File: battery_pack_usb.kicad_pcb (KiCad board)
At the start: 2 copper layers, 30.4 x 15 mm, 25 parts, among them J1 Conn_01x02_Male, J2 USB_C_Receptacle_USB2.0, SW1 SW_SPST, U1 BQ25886

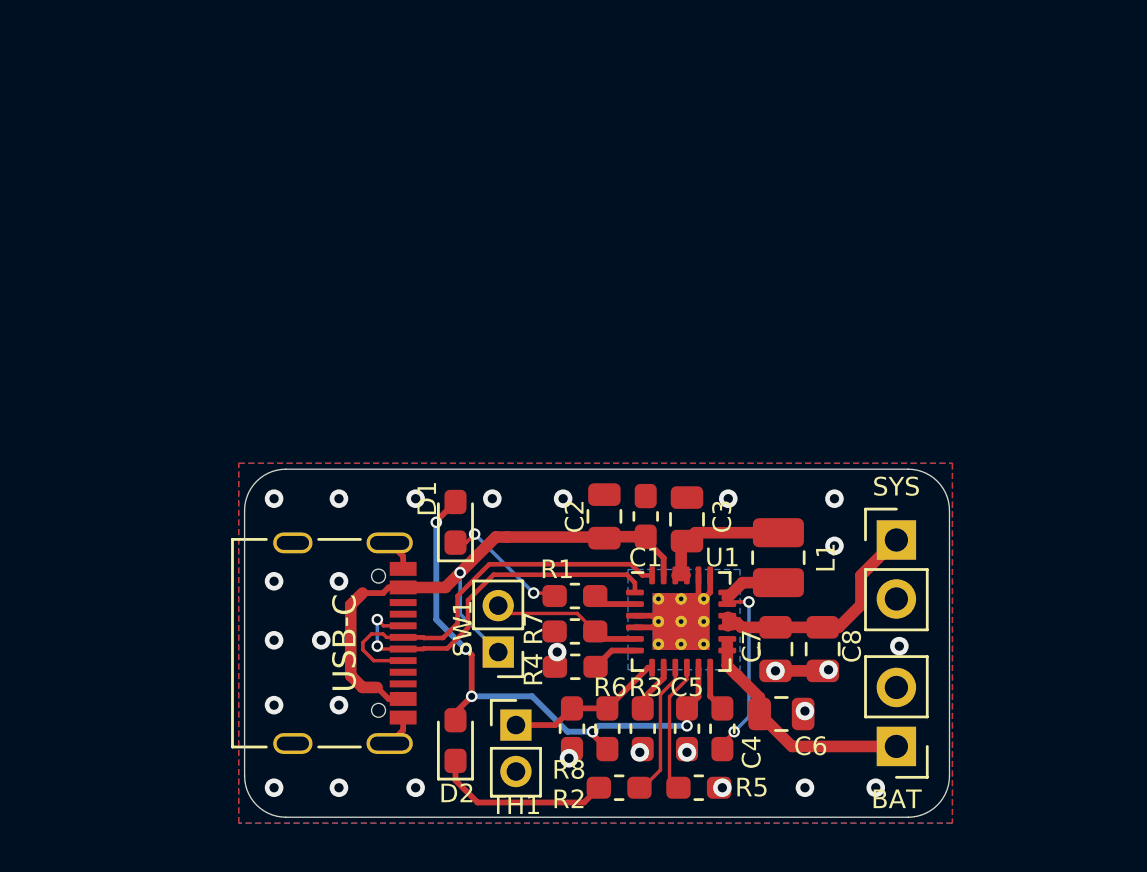
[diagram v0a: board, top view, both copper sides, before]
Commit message: Improve circuit and PCB
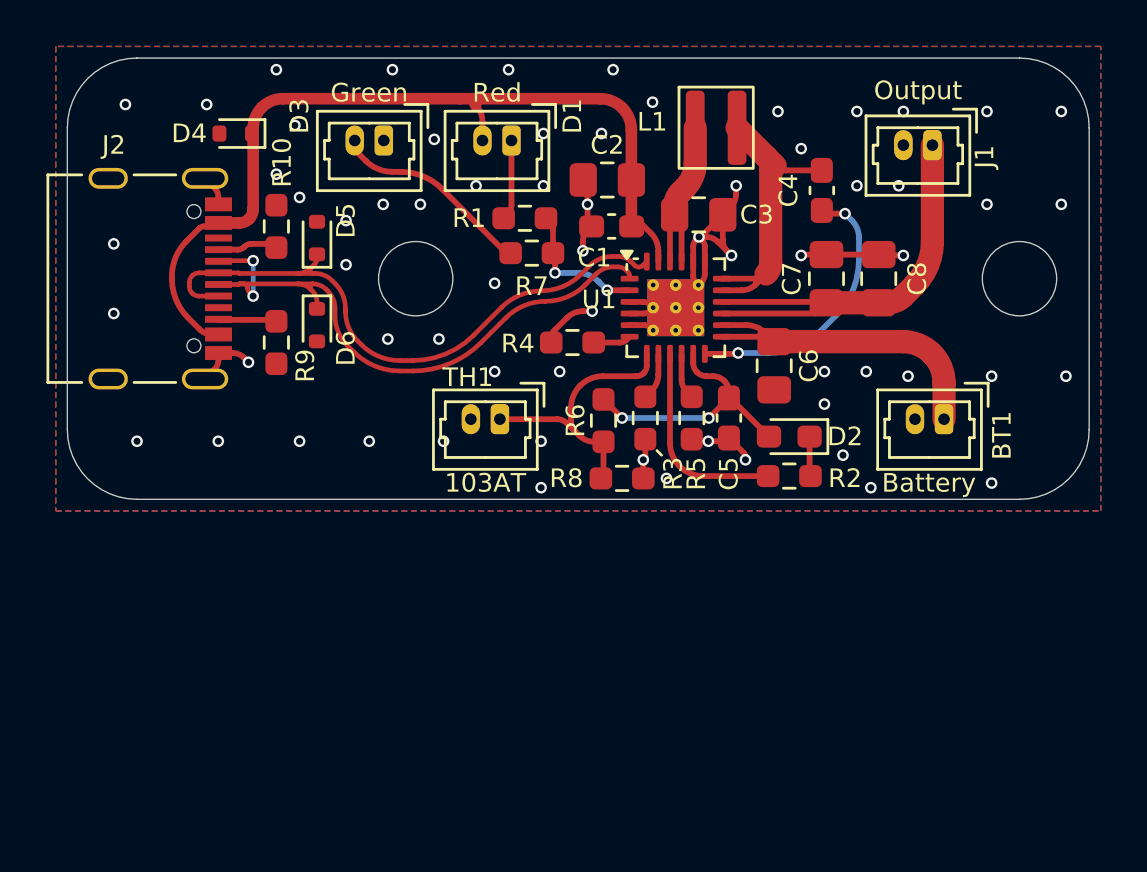
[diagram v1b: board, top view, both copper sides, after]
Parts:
- removed SW1: SW_SPST, Connector_PinHeader_2.00mm:PinHeader_1x02_P2.00mm_Vertical
- added D3: Green, Connector_Molex:Molex_PicoBlade_53047-0210_1x02_P1.25mm_Vertical, F.Cu at (109.6, 94.0)
- added D4: ESD5Zxx, Diode_SMD:D_SOD-523, F.Cu at (103.2, 93.8)
- added D5: ESD5Zxx, Diode_SMD:D_SOD-523, F.Cu at (106.8, 98.2)
- added D6: ESD5Zxx, Diode_SMD:D_SOD-523, F.Cu at (106.8, 102.0)
- added H1: MountingHole, MountingHole:MountingHole_3.2mm_M3_ISO14580, F.Cu at (111.0, 100.0)
- added H2: MountingHole, MountingHole:MountingHole_3.2mm_M3_ISO14580, F.Cu at (137.0, 100.0)
- added R10: 5k1, Resistor_SMD:R_0603_1608Metric_Pad0.98x0.95mm_HandSolder, F.Cu at (105.0, 97.8)
- added R9: 5k1, Resistor_SMD:R_0603_1608Metric_Pad0.98x0.95mm_HandSolder, F.Cu at (105.0, 102.8)
- BT1: footprint Connector_PinHeader_2.54mm:PinHeader_1x02_P2.54mm_Vertical -> Connector_Molex:Molex_PicoBlade_53047-0210_1x02_P1.25mm_Vertical
- C1: value 1u 5V -> 1u; footprint Capacitor_SMD:C_0603_1608Metric_Pad1.05x0.95mm_HandSolder -> Capacitor_SMD:C_0603_1608Metric_Pad1.08x0.95mm_HandSolder
- C2, C3: value 10u 5V -> 10u; footprint Capacitor_SMD:C_0805_2012Metric -> Capacitor_SMD:C_0805_2012Metric_Pad1.18x1.45mm_HandSolder
- C4, C5: footprint Capacitor_SMD:C_0603_1608Metric_Pad1.05x0.95mm_HandSolder -> Capacitor_SMD:C_0603_1608Metric_Pad1.08x0.95mm_HandSolder
- C6: value 10u 9V -> 10u 10V; footprint Capacitor_SMD:C_0805_2012Metric -> Capacitor_SMD:C_0805_2012Metric_Pad1.18x1.45mm_HandSolder
- C7, C8: value 22u 9V -> 22u 10V; footprint Capacitor_SMD:C_0805_2012Metric -> Capacitor_SMD:C_0805_2012Metric_Pad1.18x1.45mm_HandSolder
- D1: value LED -> Red; footprint LED_SMD:LED_0603_1608Metric_Pad1.05x0.95mm_HandSolder -> Connector_Molex:Molex_PicoBlade_53047-0210_1x02_P1.25mm_Vertical
- D2: value LED -> Blue
- J1: value Conn_01x02_Male -> Output; footprint Connector_PinHeader_2.54mm:PinHeader_1x02_P2.54mm_Vertical -> Connector_Molex:Molex_PicoBlade_53047-0210_1x02_P1.25mm_Vertical
- J2: value USB_C_Receptacle_USB2.0 -> USB_C_Receptacle_USB2.0_16P
- L1: value 1u -> 1u (XGL3515-102); footprint Inductor_SMD:L_1008_2520Metric -> extraFootprints:XxL3515
- R1, R2, R3, R4, R6, R8: footprint Resistor_SMD:R_0603_1608Metric_Pad1.05x0.95mm_HandSolder -> Resistor_SMD:R_0603_1608Metric_Pad0.98x0.95mm_HandSolder
- R5: value 7k5 -> 4k7; footprint Resistor_SMD:R_0603_1608Metric_Pad1.05x0.95mm_HandSolder -> Resistor_SMD:R_0603_1608Metric_Pad0.98x0.95mm_HandSolder
- R7: value 10k -> R; footprint Resistor_SMD:R_0603_1608Metric_Pad1.05x0.95mm_HandSolder -> Resistor_SMD:R_0603_1608Metric_Pad0.98x0.95mm_HandSolder
- TH1: footprint Connector_PinHeader_2.00mm:PinHeader_1x02_P2.00mm_Vertical -> Connector_Molex:Molex_PicoBlade_53047-0210_1x02_P1.25mm_Vertical
- moved C4 23.6 mm to (128.5, 96.2), turned to 90 degrees
- moved D2 19.4 mm to (127.1, 106.8), turned to 180 degrees
- moved L1 18.7 mm to (123.9, 93.5), turned to 0 degrees
- moved J2 17.6 mm to (100.0, 100.0)
- moved J1 17.1 mm to (133.2, 94.2), turned to 180 degrees
- moved D1 16.6 mm to (115.1, 94.0), turned to 180 degrees
- moved R1 16.4 mm to (115.7, 97.4), turned to 180 degrees
- moved R7 16.4 mm to (116.0, 98.9)
- moved C8 16.1 mm to (130.9, 100.0), turned to 90 degrees
- moved C7 16.1 mm to (128.7, 100.0), turned to 90 degrees
- moved R5 15.9 mm to (122.9, 106.0), turned to 90 degrees
- moved R2 15.3 mm to (127.1, 108.5), turned to 180 degrees
- moved C6 15.0 mm to (126.4, 103.8), turned to -90 degrees
- moved C2 14.5 mm to (119.2, 95.8), turned to 180 degrees
- moved BT1 14.2 mm to (133.8, 106.0)
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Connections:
- net /SYS renamed Net-(J1-Pin_1)
- C1 pad 1: GND -> /V_{Bus}
- C1 pad 2: Net-(SW1-A) -> GND
- C2 pad 1: GND -> /V_{Bus}
- C2 pad 2: Net-(SW1-A) -> GND
- D1 pad 2: /REGN -> /V_{Bus}
- J2 pad A4: Net-(SW1-A) -> /V_{Bus}
- J2 pad A5: unconnected-(J2-CC1-PadA5) -> Net-(J2-CC1)
- J2 pad A9: Net-(SW1-A) -> /V_{Bus}
- J2 pad B4: Net-(SW1-A) -> /V_{Bus}
- J2 pad B5: unconnected-(J2-CC2-PadB5) -> Net-(J2-CC2)
- J2 pad B9: Net-(SW1-A) -> /V_{Bus}
- R1 pad 1: Net-(D1-K) -> Net-(U1-STAT)
- R1 pad 2: Net-(U1-STAT) -> Net-(D1-K)
- R7 pad 1: Net-(SW1-B) -> Net-(U1-STAT)
- R7 pad 2: GND -> Net-(D3-A)
- U1 pad 23: Net-(SW1-A) -> /V_{Bus}
- U1 pad 5: Net-(SW1-B) -> GND
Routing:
- net /V_{Bus}: track 0.00 -> 37.9 mm
- net Net-(SW1-A): track 25.8 -> 0.00 mm, vias 1 -> 0
- net GND: track 12.0 -> 29.7 mm, vias 28 -> 65
- net /REGN: track 24.4 -> 10.8 mm, vias 5 -> 2
- net /D-: track 16.1 -> 27.2 mm
- net Net-(U1-BTST): track 1.97 -> 11.9 mm, vias 0 -> 2
- net /D+: track 17.1 -> 26.8 mm
- net Net-(J1-Pin_1): track 10.1 -> 18.8 mm
- net Net-(D3-A): track 0.00 -> 8.17 mm
- net Net-(SW1-B): track 6.48 -> 0.00 mm
- net Net-(D2-K): track 7.67 -> 1.66 mm
- net Net-(U1-TS): track 6.89 -> 12.3 mm
- net Net-(U1-ICHGSET): track 5.64 -> 1.69 mm
- net Net-(U1-STAT): track 1.85 -> 5.42 mm, vias 0 -> 2
- net BAT: track 10.2 -> 13.4 mm
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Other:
- board size 30.4 x 15 mm -> 44 x 19 mm
- rule pad_to_mask_clearance: 0.05 -> 0
- board text added: "2S USB-C Li-Ion charger v1.1 2024-06 by MG-5"
- board text added: "JLCJLCJLCJLC"
- board text removed: "2S-USB-Charger V1.0 by MG 2020-08"
